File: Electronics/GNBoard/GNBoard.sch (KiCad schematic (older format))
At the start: 57 parts, among them K1 IR1, K10 IR4, K11 CNY_1, K12 CNY_2, K13 CNY_3, K14 CNY_4, K2 IR2, K3 SERVO_1, K4 SERVO_2, K5 SERVO_3, K6 SERVO_4, K7 SERVO_5, K9 IR3, M1 XBEE, P1 Battery, P10 Nose_Heater, P11 CONN_1, P2 LDR_1, P3 Spk, P4 I2C_1, P5 LDR_2, P6 DHT_Conn, P7 LDR_3, P8 LDR_4, P9 Nose_Sense, Q1 NPN, SW1 PowerSwitch, SW2 SW_PUSH, SW3 SW_PUSH, U1 LM2576

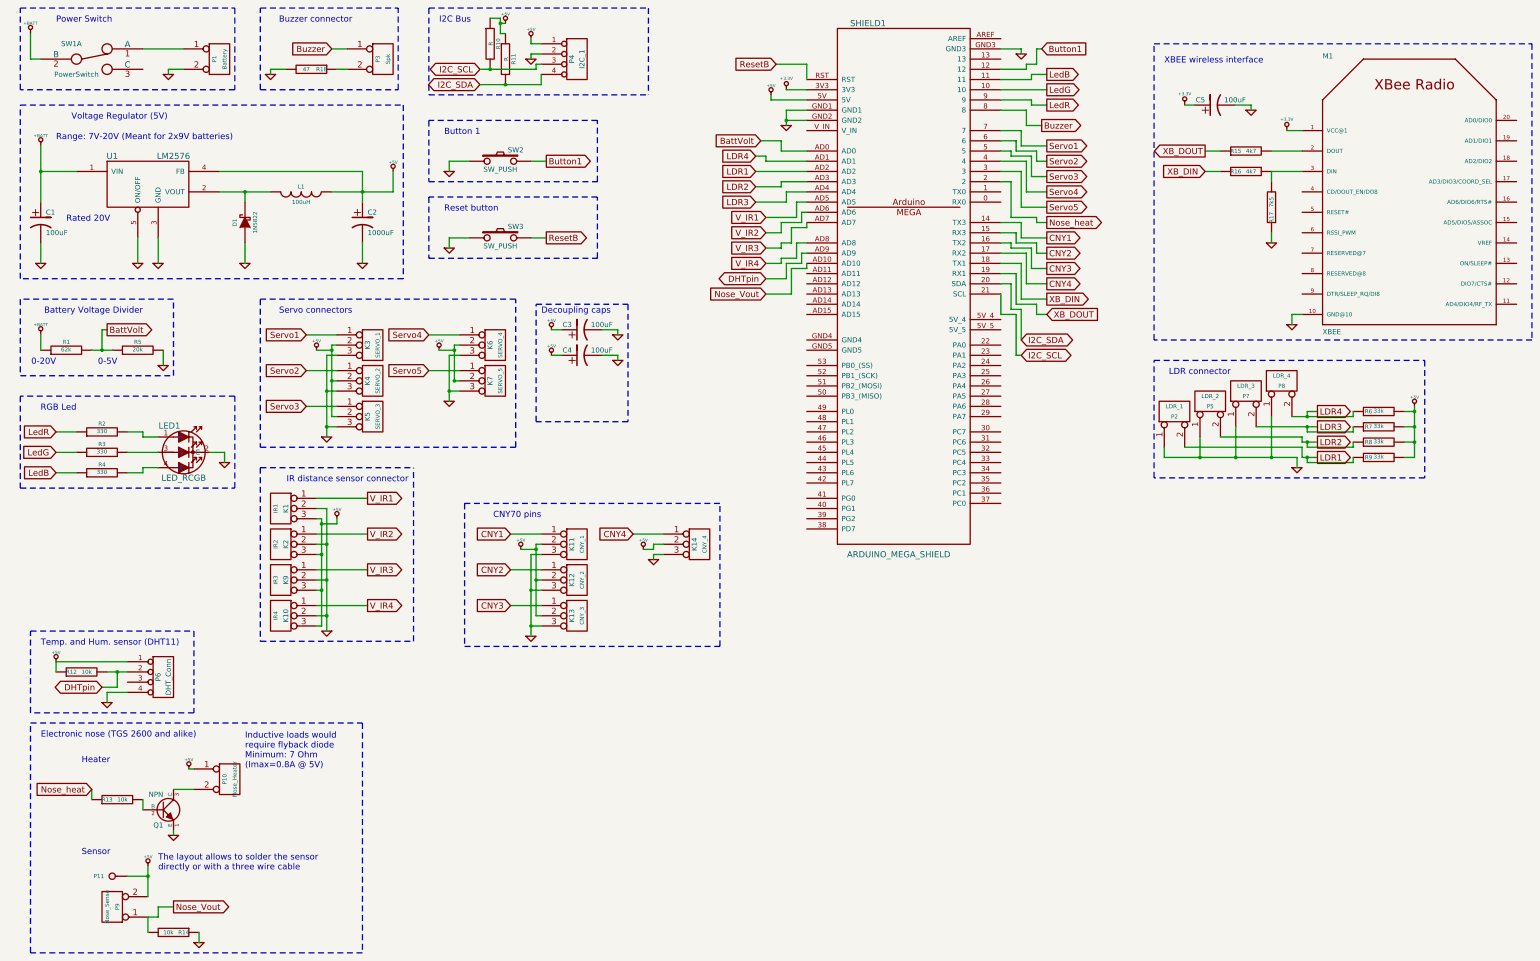
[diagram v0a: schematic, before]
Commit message: Finished v1.0 of the GNBoard
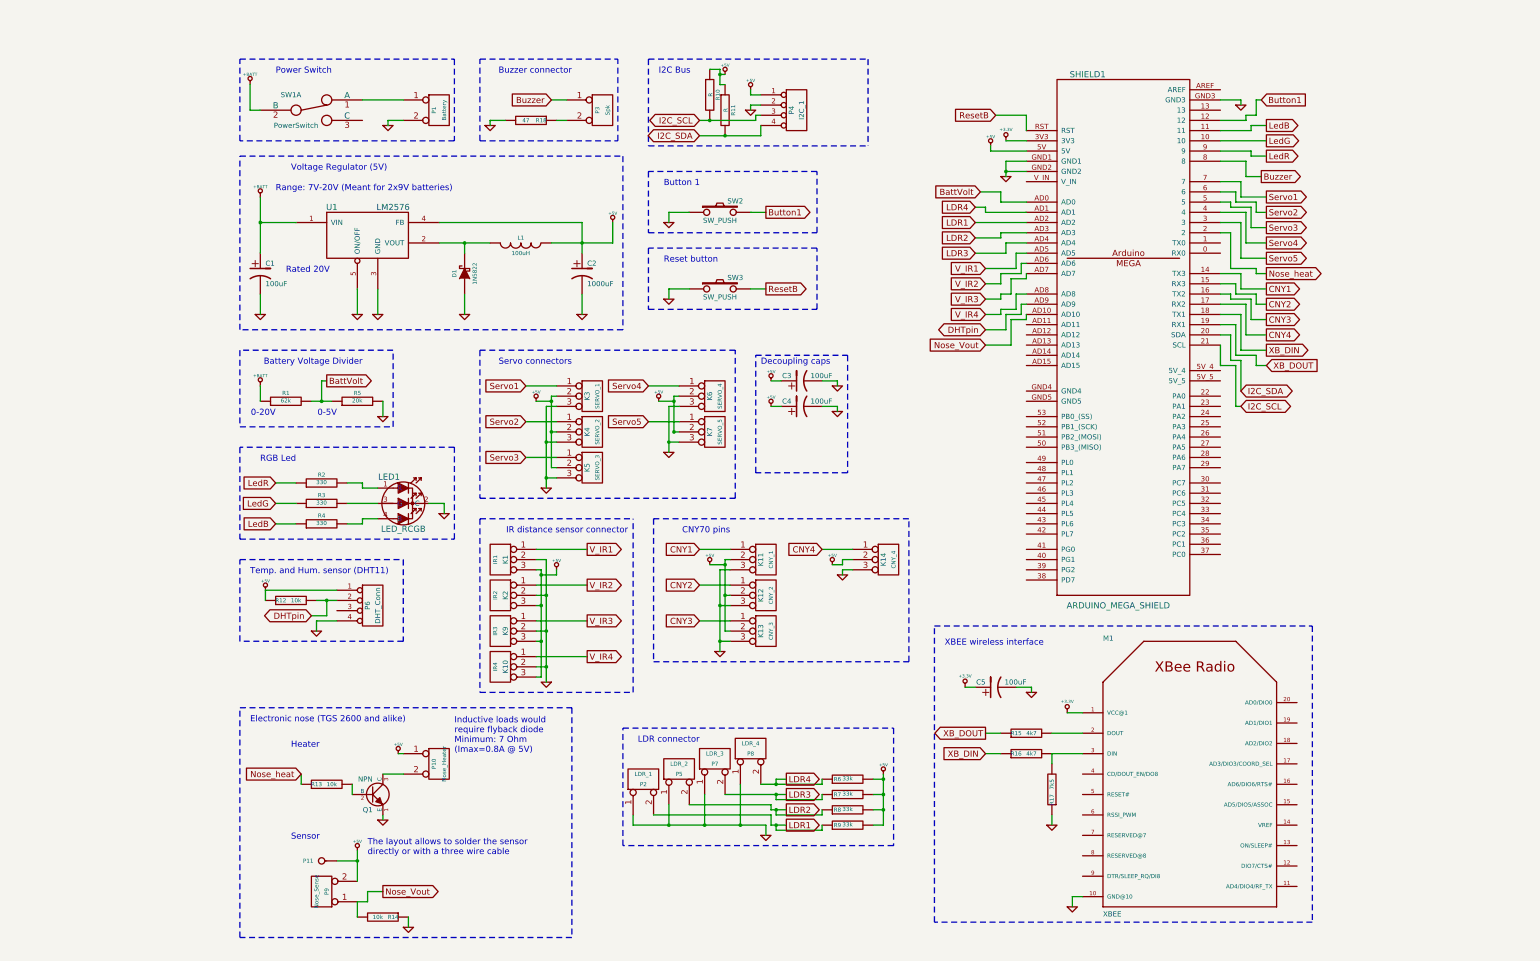
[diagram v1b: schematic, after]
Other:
- moved on the sheet: C1, C2, C3, C4, C5, D1, K1, K10, K11, K12, K13, K14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
